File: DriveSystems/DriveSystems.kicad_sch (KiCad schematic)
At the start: 22 parts, among them J1 Raspberry_Pi_4, M1 Motor_Servo, M2 Motor_Servo, SW1 SW_Rotary_1x2_MP, U1 RoboClaw Motor Controller, U2 5304 Gear Motor, U3 24VDC UBC-C PSU, U4 24V 5V10A DCDC Stepdown, U5 RoboClaw VClamp, U6 Pwr Res

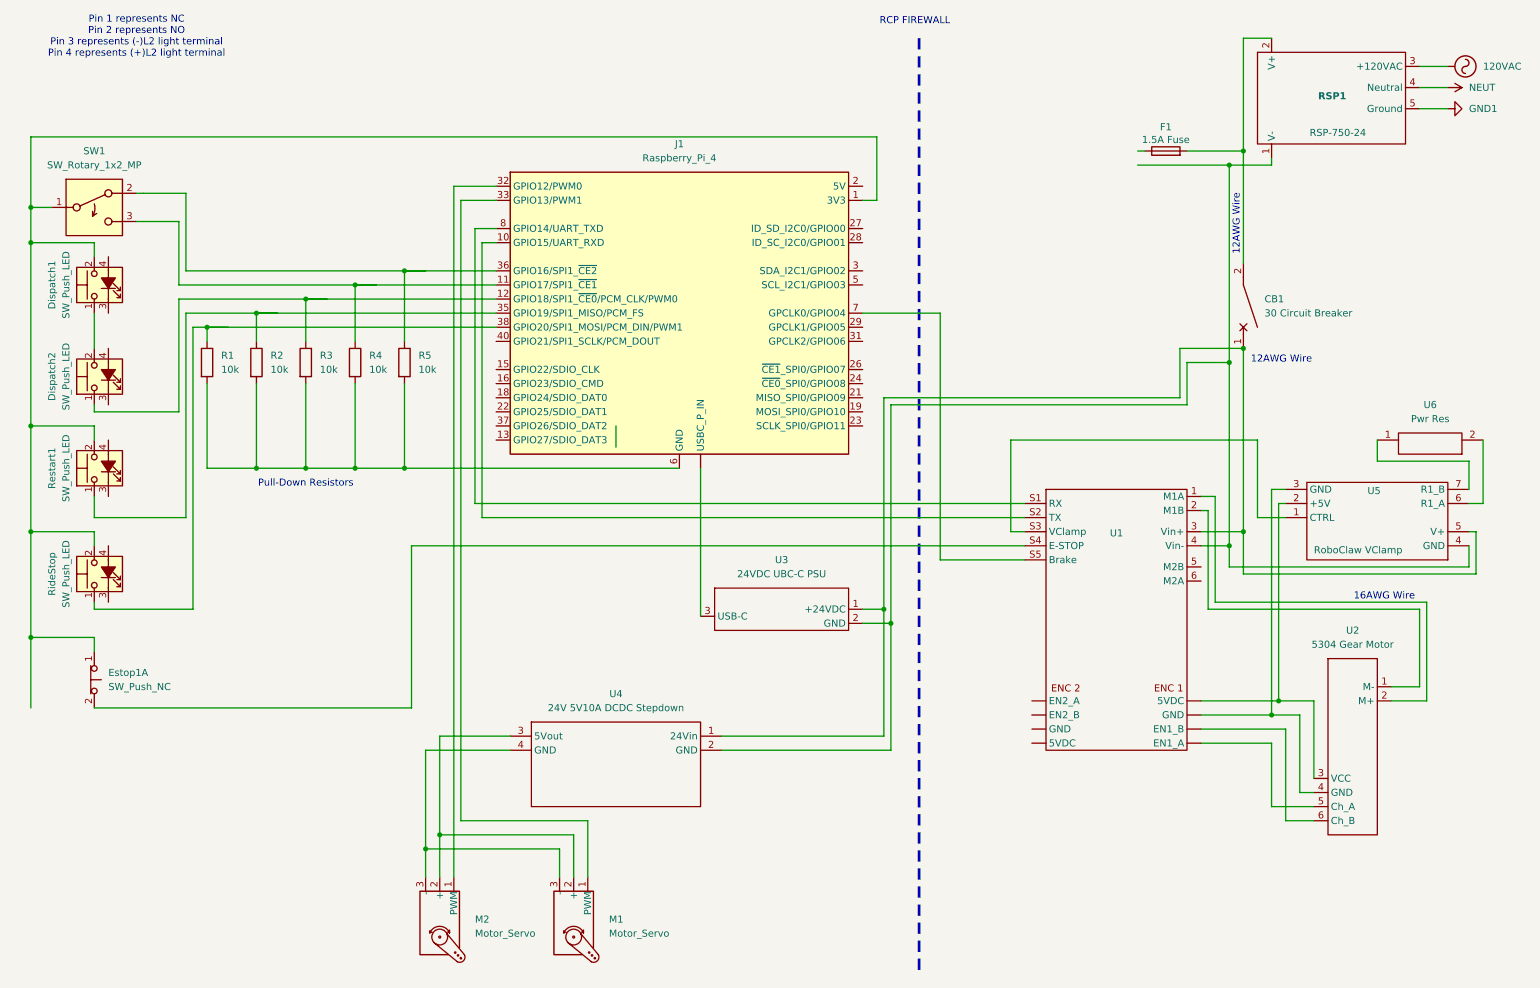
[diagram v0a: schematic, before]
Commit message: Update DriveSystems.kicad_sch
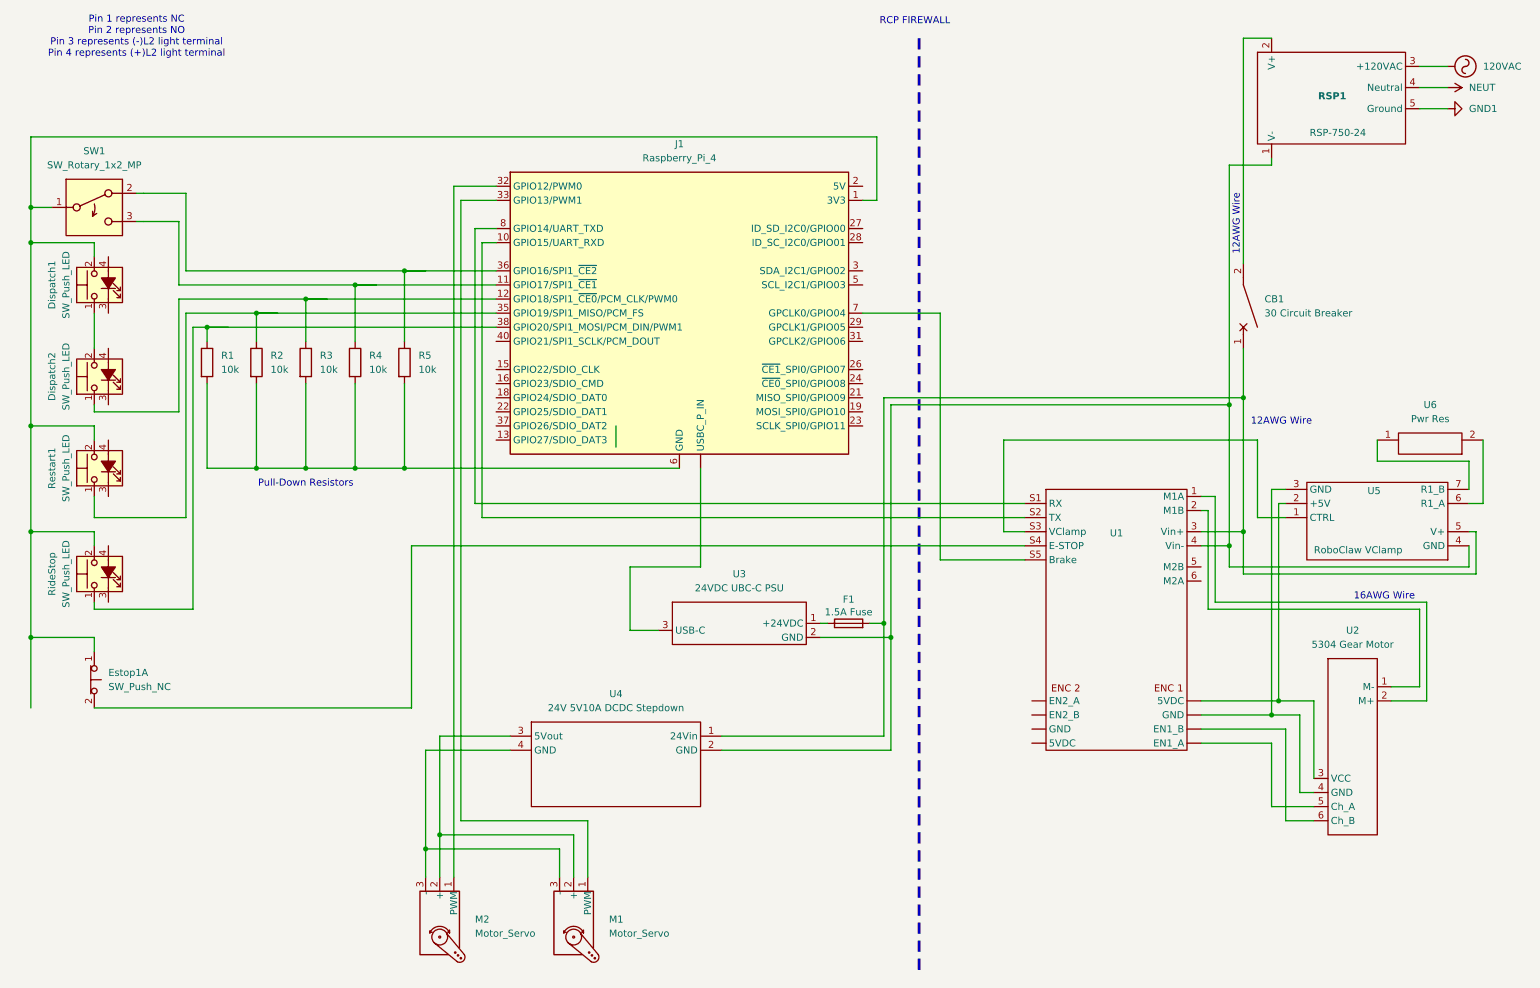
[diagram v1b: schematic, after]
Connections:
- net at U1. (EN1_A): now also U2.6 (Ch_B)
- net at CB1.1, U1.3 (Vin+), U4.1 (24Vin)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: now also F1.2; no longer U3.1 (+24VDC)
- net at F1.1: now also U3.1 (+24VDC)
- net at CB1.2: no longer F1.2
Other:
- moved on the sheet: F1, U3
